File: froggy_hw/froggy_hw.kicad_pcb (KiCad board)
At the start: 2 copper layers, 100 x 100 mm, 196 parts, among them J1 I2C, J10 M4, J11 M4, J12 POWER_OUT, J13 NTC, J14 VALVE, J15 NOZZLE, J16 FAN, J17 FAN, J18 LED, J2 SWD, J3 Power_DMX_IO, J4 USB_C, J5 NC3FAAH, J6 NC3MAAH-0, J7 M4, J8 M4, J9 M4, P1 TC2030_STM32, Q10 AON6262E, Q11 AON6262E, Q12 AO3400A, Q13 AO3400A, Q14 AO3401A, Q15 AO3401A, Q16 AO3400A, Q17 AO3400A, Q4 S8050, Q5 S8050, Q6 S8050, Q7 S8550, Q8 S8050, Q9 S8550, SW1 SW_Push, U1 STM32F030F4Px, U10 SY8303AIC, U2 SN75176AD, U3 TLP2361, U4 TLP2361, U5 TLP2361, U6 B0505S-1WR3, U7 STUSB4500, U8 SY8303AIC, U9 SY8303AIC

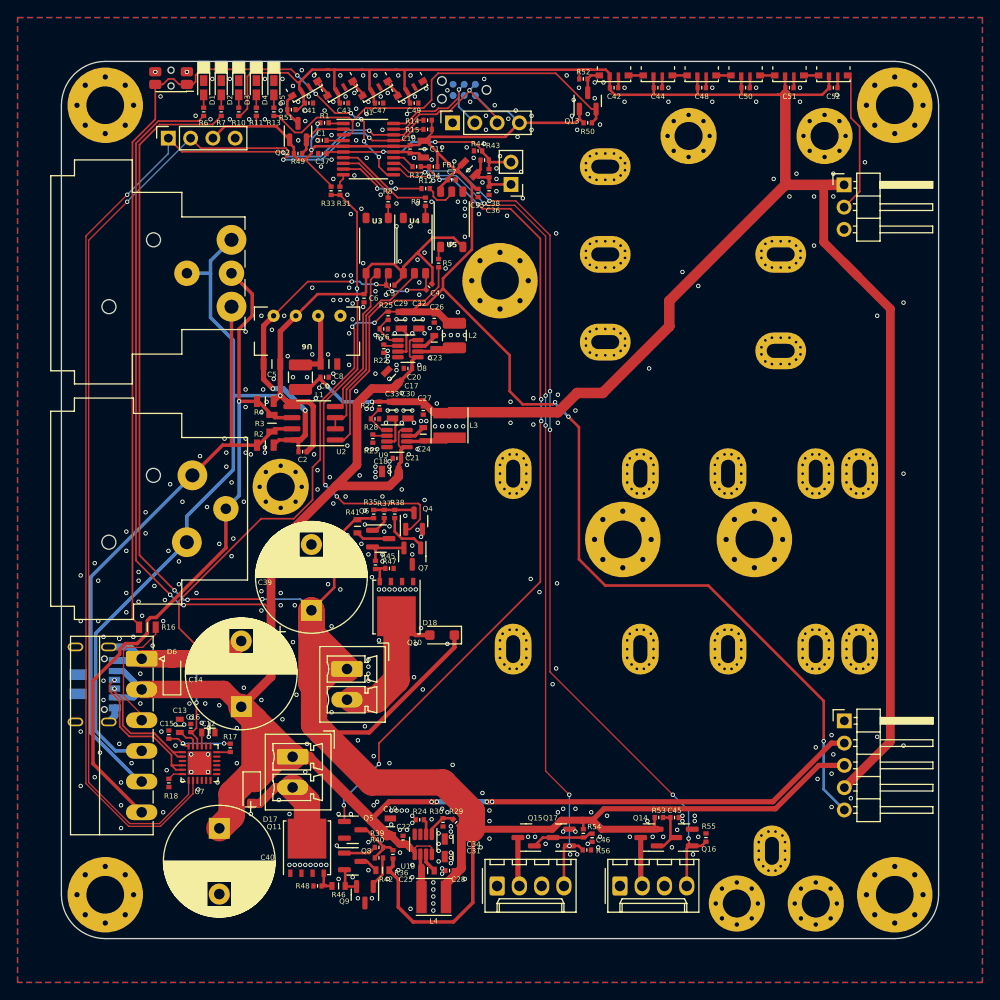
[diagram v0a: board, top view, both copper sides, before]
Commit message: moved to esp32
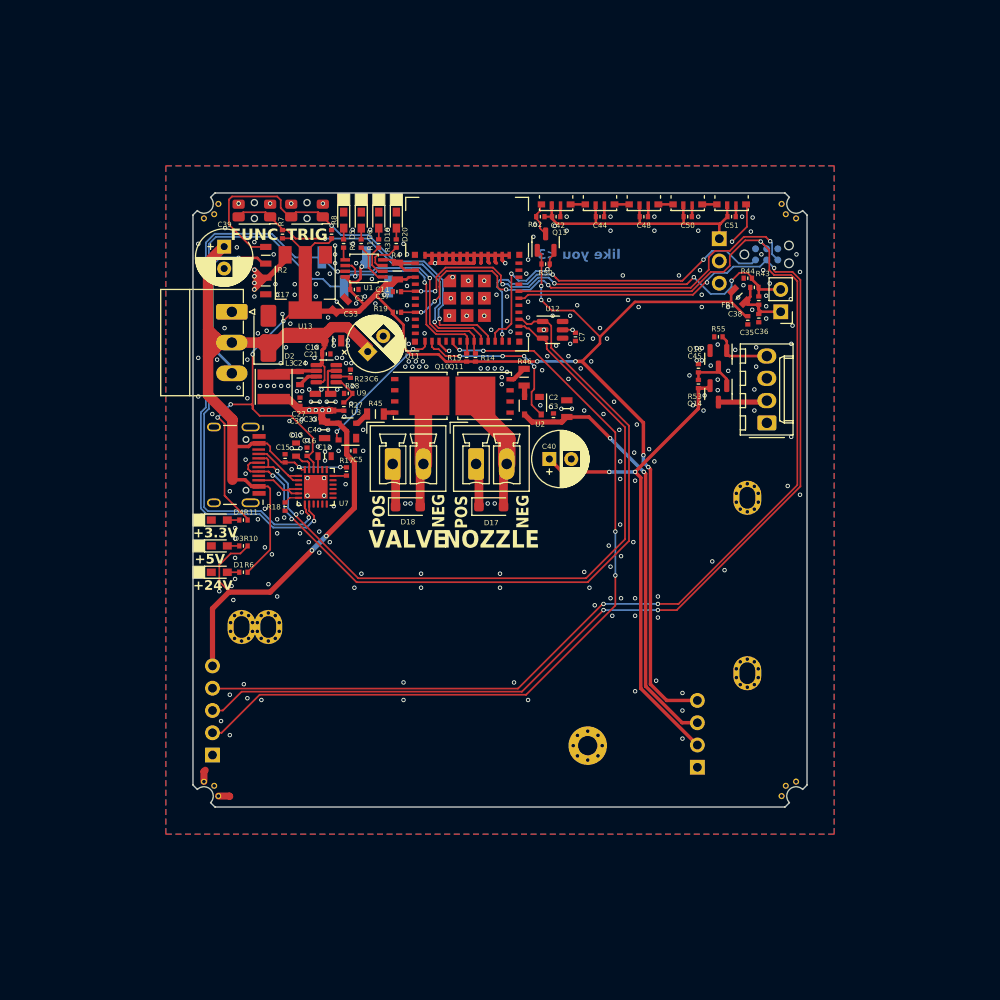
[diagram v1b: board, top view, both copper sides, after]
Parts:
- removed C10, C20, C22, C26, C28, C41, C43, C46, C47, C49, C52, C9: 100n, otter:C_0402
- removed C14: 100u, Capacitor_THT:CP_Radial_D12.5mm_P7.50mm
- removed C19, C29, C31, C32, C34, C8: 4u7, otter:C_0805
- removed C23, C25: 100n, otter:C_0603
- removed D11, D13, D16, D7, D9: SK6805-SIDE-G, otter:SK6805-SIDE-G
- removed the G*** at (100.0, 109.5)
- removed L1, L2: 4u7, Inductor_SMD:L_1210_3225Metric
- removed L4: 4u7, Inductor_SMD:L_Taiyo-Yuden_MD-4040
- removed P1: TC2030_STM32, otter:TC2030
- removed Q12, Q17: AO3400A, Package_TO_SOT_SMD:SOT-23
- removed Q15: AO3401A, Package_TO_SOT_SMD:SOT-23
- removed Q4, Q5, Q6, Q8: S8050, Package_TO_SOT_SMD:SOT-23
- removed Q7, Q9: S8550, Package_TO_SOT_SMD:SOT-23
- removed R12, R37, R38, R39, R40, R9: 200, otter:R_0402
- removed R13, R30, R33, R34, R35, R36, R47, R48, R49, R51, R56: 5k1, otter:R_0402
- removed R16: 133, otter:R_0805
- removed R22, R24, R26, R54: 22k, otter:R_0402
- removed R25, R29: 100k, otter:R_0402
- removed R31, R32: 0, otter:R_0402
- removed R41, R42: 20, otter:R_0603
- removed REF** (x16): pad_1.6_3.2, otter:pad_1.6_3.2
- removed REF** (x5): MountingHole_3.2mm_M3_Pad_Via, MountingHole:MountingHole_3.2mm_M3_Pad_Via
- removed REF** (x2): MountingHole_4.3mm_M4_Pad_Via, MountingHole:MountingHole_4.3mm_M4_Pad_Via
- removed U10, U8: SY8303AIC, Package_TO_SOT_SMD:TSOT-23-8
- removed U4, U5: TLP2361, otter:TLP2361
- removed U6: B0505S-1WR3, otter:B0303S-1WR3
- added C53: 4u7, otter:C_0805, F.Cu at (81.8, 77.8)
- added D19: HEAT, otter:LED_0603_1608Metric, F.Cu at (86.2, 68.1)
- added D20: ERR, otter:LED_0603_1608Metric, F.Cu at (88.2, 68.1)
- added G***: LOGO, LOGO, B.Cu at (116.4, 71.2)
- added G***: LOGO, LOGO, B.Cu at (100.0, 108.5)
- added J19: HOTEND, otter:froggy_PAD, F.Cu at (70.5, 114.5)
- added P2: TC2030-CTX-Tag-Connect-ESP32, otter:TC2030, B.Cu at (130.4, 72.0)
- added R19: 5k1, otter:R_0402, F.Cu at (88.2, 78.6)
- added SW2: SW_Push, Button_Switch_SMD:SW_SPST_EVQP7C, F.Cu at (78.0, 67.0)
- added U11: ESP32-C3-MINI-1, otter:ESP32-C3-MINI-1, F.Cu at (96.2, 77.0)
- added U12: USBLC6-4, Package_TO_SOT_SMD:SOT-23-6, F.Cu at (106.0, 80.6)
- added U13: AMS1117-3.3, Package_TO_SOT_SMD:SOT-223-3_TabPin2, F.Cu at (77.8, 75.2)
- C2, C4: value 100n -> 4u7; footprint otter:C_0402 -> otter:C_0805
- C39, C40: footprint Capacitor_THT:CP_Radial_D12.5mm_P7.50mm -> Capacitor_THT:CP_Radial_D6.3mm_P2.50mm
- C5: value 4u7 -> 100n; footprint otter:C_0805 -> otter:C_0402
- C6: value DNP -> 100u; footprint otter:C_0402 -> Capacitor_THT:CP_Radial_D6.3mm_P2.50mm
- D1: value 12V -> 24V
- D2: value 12V -> D210; footprint otter:LED_0603_1608Metric -> Diode_SMD:D_SMA
- D6: value D210 -> OK; footprint Diode_SMD:D_SOD-123F -> otter:LED_0603_1608Metric
- J1: footprint otter:PinSocket_1x04_P2.54mm_Vertical_center -> Connector_PinHeader_2.54mm:PinHeader_1x04_P2.54mm_Vertical_SMD_Pin1Left; moved to B.Cu
- J10, J11: value M4 -> MOUNT; footprint MountingHole:MountingHole_4.3mm_M4_Pad_Via -> MountingHole:MountingHole_2.2mm_M2_Pad_Via
- J12: value POWER_OUT -> MOUNT; footprint Connector_PinHeader_2.54mm:PinHeader_1x05_P2.54mm_Horizontal -> MountingHole:MountingHole_2.2mm_M2_Pad_Via
- J17: value FAN -> MOUNT; footprint Connector_Molex:Molex_KK-254_AE-6410-04A_1x04_P2.54mm_Vertical -> MountingHole:MountingHole_2.2mm_M2_Pad_Via
- J18: moved to B.Cu
- J2: value SWD -> POWER; footprint otter:PinSocket_1x04_P2.54mm_Vertical_center -> Connector_Phoenix_MC:PhoenixContact_MC_1,5_3-G-3.5_1x03_P3.50mm_Horizontal
- J3: value Power_DMX_IO -> DMX CARD; footprint Connector_Phoenix_MC:PhoenixContact_MC_1,5_6-G-3.5_1x06_P3.50mm_Horizontal -> MountingHole:MountingHole_2.2mm_M2_Pad_Via
- J4: value USB_C -> USB; footprint otter:USB-C_Power -> otter:USB-C 16Pin; moved to F.Cu
- J5: value NC3FAAH -> POWER_OUT; footprint Connector_Audio:Jack_XLR_Neutrik_NC3FAAH_Horizontal -> Connector_PinHeader_2.54mm:PinHeader_1x04_P2.54mm_Horizontal; moved to B.Cu
- J6: value NC3MAAH-0 -> DMX; footprint Connector_Audio:Jack_XLR_Neutrik_NC3MAAH-0_Horizontal -> Connector_PinHeader_2.54mm:PinHeader_1x05_P2.54mm_Horizontal; moved to B.Cu
- J7, J8, J9: value M4 -> HOTEND; footprint MountingHole:MountingHole_4.3mm_M4_Pad_Via -> otter:froggy_PAD
- R1, R5: value 200 -> 22k
- R10, R11: value 5k1 -> 22k
- R2: value 580 -> 133
- R3: value 133 -> 22k; footprint otter:R_0805 -> otter:R_0402
- R4: value 580 -> 22k; footprint otter:R_0805 -> otter:R_0402
- R44: value 100k -> 5k1
- R45: footprint otter:R_0402 -> otter:R_0805
- R46: footprint otter:R_0603 -> otter:R_0805
- R6: value 22k -> 100k
- R7: value 13k -> 5k1
- R8: value 200 -> 5k1
- U1: value STM32F030F4Px -> PCA9536DP; footprint Package_SO:TSSOP-20_4.4x6.5mm_P0.65mm -> Package_SO:TSSOP-8_3x3mm_P0.65mm
- U2: value SN75176AD -> MIC4416YM4; footprint Package_SO:SOIC-8_3.9x4.9mm_P1.27mm -> Package_TO_SOT_SMD:SOT-143
- U3: value TLP2361 -> MIC4416YM4; footprint otter:TLP2361 -> Package_TO_SOT_SMD:SOT-143
- moved J8 97.7 mm to (128.2, 119.7)
- moved J12 93.8 mm to (66.2, 66.2)
- moved J5 63.6 mm to (122.5, 130.5), turned to 0 degrees
- moved R46 61.7 mm to (102.8, 86.0), turned to 90 degrees
- moved J6 58.8 mm to (67.2, 129.1), turned to 0 degrees
- moved R55 57.1 mm to (124.9, 81.4), turned to 0 degrees
- moved C40 56.5 mm to (105.6, 95.3), turned to 0 degrees
- moved D6 56.2 mm to (84.2, 68.1), turned to -90 degrees
- moved J16 55.4 mm to (130.4, 91.2), turned to 90 degrees
- moved Q11 55.4 mm to (98.2, 88.1), turned to 180 degrees
- moved D1 55.3 mm to (68.0, 108.2), turned to 0 degrees
- moved Q16 54.7 mm to (124.9, 83.9), turned to -90 degrees
- moved R6 52.7 mm to (70.8, 108.2), turned to 180 degrees
- moved D3 52.3 mm to (68.0, 105.2), turned to 0 degrees
- moved J3 51.8 mm to (110.0, 128.0), turned to 0 degrees
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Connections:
- C1 pad 1: Net-(U1-NRST) -> +3V3
- C15 pad 1: VBUS -> +24V
- C17 pad 2: +24V -> +5V
- C2 pad 1: RS485_GND -> GND
- C2 pad 2: Net-(U2-VCC) -> +5V
- C3 pad 1: RS485_GND -> GND
- C3 pad 2: Net-(U2-VCC) -> +5V
- C39 pad 1: +12V -> +24V
- C4 pad 1: RS485_GND -> GND
- C4 pad 2: Net-(U2-VCC) -> +5V
- C5 pad 1: RS485_GND -> GND
- C5 pad 2: Net-(U2-VCC) -> +5V
- C6 pad 1: GND -> +24V
- C6 pad 2: RS485_GND -> GND
- C7 pad 1: GND -> +5V
- C7 pad 2: +3V3 -> GND
- D18 pad 1: +12V -> +24V
- D2 pad 1: GND -> +24V
- D2 pad 2: Net-(D2-A) -> GND
- D6 pad 1: +24V -> GND
- D6 pad 2: GND -> Net-(D6-A)
- J1 pad 1: SDA -> GND
- J1 pad 2: SCL -> +3V3
- J1 pad 3: +3V3 -> SCL
- J1 pad 4: GND -> SDA
- J14 pad 1: +12V -> +24V
- J16 pad 4: FAN_1 -> /Out/FAN_1
- J18 pad 2: Net-(D16-DOUT) -> Net-(D15-DOUT)
- J2 pad 2: SWCLK -> +24V
- J2 pad 3: SWDIO -> Net-(J2-Pin_3)
- J5 pad 1: RS485_GND -> GND
- J5 pad 2: RS485_B -> +24V
- J5 pad 3: RS485_A -> +5V
- J6 pad 1: RS485_GND -> GND
- J6 pad 2: RS485_B -> RS485_DE
- J6 pad 3: RS485_A -> ESP32_RXD
- Q13 pad 2: LED_1 -> LED_0
- Q14 pad 2: +12V -> +24V
- Q16 pad 1: FAN_1 -> /Out/FAN_1
- R1 pad 1: +3V3 -> Net-(U1-IO0)
- R1 pad 2: Net-(U1-BOOT0) -> Net-(D6-A)
- R17 pad 2: VBUS -> +24V
- R2 pad 1: RS485_B -> Net-(J2-Pin_3)
- R2 pad 2: Net-(U2-VCC) -> IO
- R3 pad 1: RS485_A -> Net-(U1-IO1)
- R3 pad 2: RS485_B -> Net-(D19-A)
- R4 pad 1: RS485_GND -> Net-(U1-IO2)
- R4 pad 2: RS485_A -> Net-(D20-A)
- R45 pad 1: Net-(Q6-E) -> Net-(U3-GATE)
- R46 pad 1: Net-(Q8-E) -> Net-(U2-GATE)
- R5 pad 1: Net-(U2-R) -> Net-(U1-IO3)
- R5 pad 2: Net-(U5-A) -> Net-(D5-A)
- R50 pad 2: LED_1 -> LED_0
- R53 pad 2: +12V -> +24V
- R55 pad 2: FAN_1 -> /Out/FAN_1
- R7 pad 1: +12V -> Net-(U11-IO6)
- R7 pad 2: Net-(D2-A) -> +3V3
- R8 pad 1: Net-(U3-A) -> IO
- R8 pad 2: RS485_TX -> +3V3
- SW1 pad 1: IO -> Net-(U11-IO6)
- U1 pad 1: Net-(U1-BOOT0) -> Net-(U1-IO0)
- U1 pad 2: LED_0 -> Net-(U1-IO1)
- U1 pad 3: LED_1 -> Net-(U1-IO2)
- U1 pad 4: Net-(U1-NRST) -> GND
- U1 pad 5: +3V3 -> Net-(U1-IO3)
- U1 pad 6: NTC -> SCL
- U1 pad 7: RS485_DE -> SDA
- U1 pad 8: RS485_TX -> +3V3
- U2 pad 1: Net-(U2-R) -> GND
- U2 pad 2: Net-(U2-DE) -> Net-(U2-GATE)
- U2 pad 3: Net-(U2-DE) -> +5V
- U2 pad 4: Net-(U2-D) -> NOZZLE
- U3 pad 1: Net-(U3-A) -> GND
- U3 pad 3: GND -> +5V
- U3 pad 4: RS485_GND -> VALVE
- U7 pad 24: VBUS -> +24V
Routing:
- net +12V: track 257.9 -> 0.00 mm, vias 3 -> 0
- net ESP32_TXD: track 0.00 -> 138.7 mm, vias 0 -> 3
- net ESP32_RXD: track 0.00 -> 136.3 mm, vias 0 -> 4
- net RS485_GND: track 133.4 -> 0.00 mm, vias 1 -> 0
- net FAN_1: track 105.4 -> 0.00 mm, vias 6 -> 0
- net +24V: track 273.2 -> 171.4 mm, vias 6 -> 4
- net FAN_2: track 98.0 -> 0.00 mm, vias 6 -> 0
- net Net-(Q5-B): track 93.9 -> 0.00 mm, vias 6 -> 0
- net USB_D+: track 0.00 -> 86.7 mm, vias 0 -> 2
- net RS485_DE: track 11.2 -> 94.7 mm, vias 0 -> 4
- net USB_D-: track 0.00 -> 82.8 mm, vias 0 -> 2
- net RS485_A: track 80.2 -> 0.00 mm, vias 1 -> 0
- net RS485_B: track 71.6 -> 0.00 mm
- net +3V3: track 262.9 -> 194.4 mm, vias 9 -> 11
- net ESP32_EN: track 0.00 -> 53.6 mm, vias 0 -> 5
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- added copper zone on In1.Cu, net +24V
- added copper zone on In2.Cu, net +24V
- added copper zone on In1.Cu, net GND
- added copper zone on In2.Cu, net GND
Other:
- board size 100 x 100 mm -> 70 x 70 mm
- copper layers 2 -> 4
- board text added: "DE"
- board text added: "ERROR"
- board text added: "HEAT"
- board text added: "OK"
- board text added: "POWER"
- board text added: "RXD"
- board text added: "TRIG"
- board text added: "TXD"
- board text added: "[CAUTION] [HOT]"
- board text added: "by fiona & Jana | v1.1.0 - 2024 | github.com/Jana-Marie/foxtruder/"
- board text added: "like you <3"
- board text removed: "A"
- board text removed: "B"
- board text removed: "DATA"
- board text removed: "FAULT"
- board text removed: "READY"
- board text removed: "STATUS"
- board text removed: "SWCLK"
- board text removed: "SWDIO"
